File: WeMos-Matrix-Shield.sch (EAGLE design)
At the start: 16 parts, among them CN1 1X4-BIG, J2 POWER_JACKPTH, U1 LDR, U2 DS18B20, X1 SPTAF_25.0MM

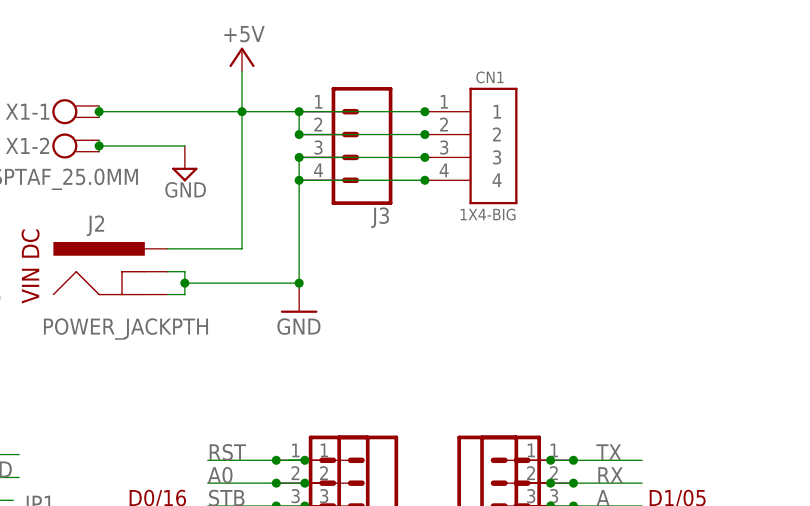
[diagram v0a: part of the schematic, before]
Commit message: Updated to V1.5
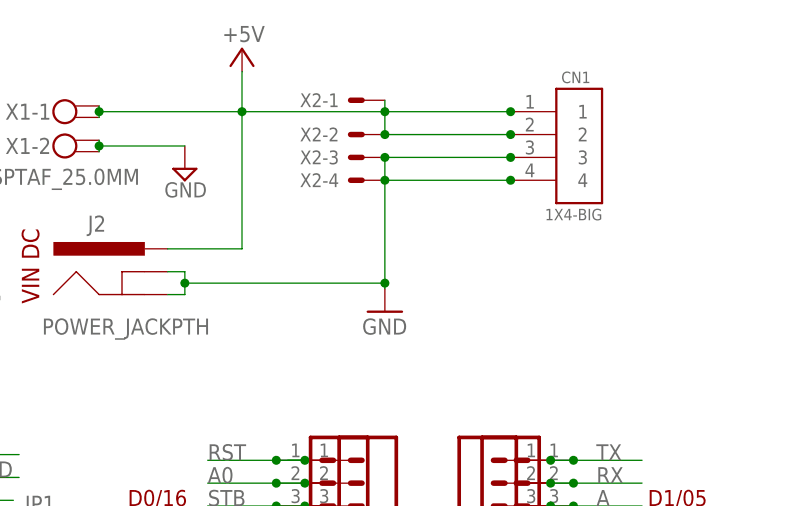
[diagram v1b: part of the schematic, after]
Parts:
- removed J3: (no value), SparkFun-Connectors:CONN_04SCREW
- added X2: (no value), con-molex:KK-156-4
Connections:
- net 5V: now also X2-1.S, X2-2.S; no longer J3.1, J3.2
- net GND: now also X2-3.S, X2-4.S; no longer J3.3, J3.4
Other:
- moved on the sheet: CN1

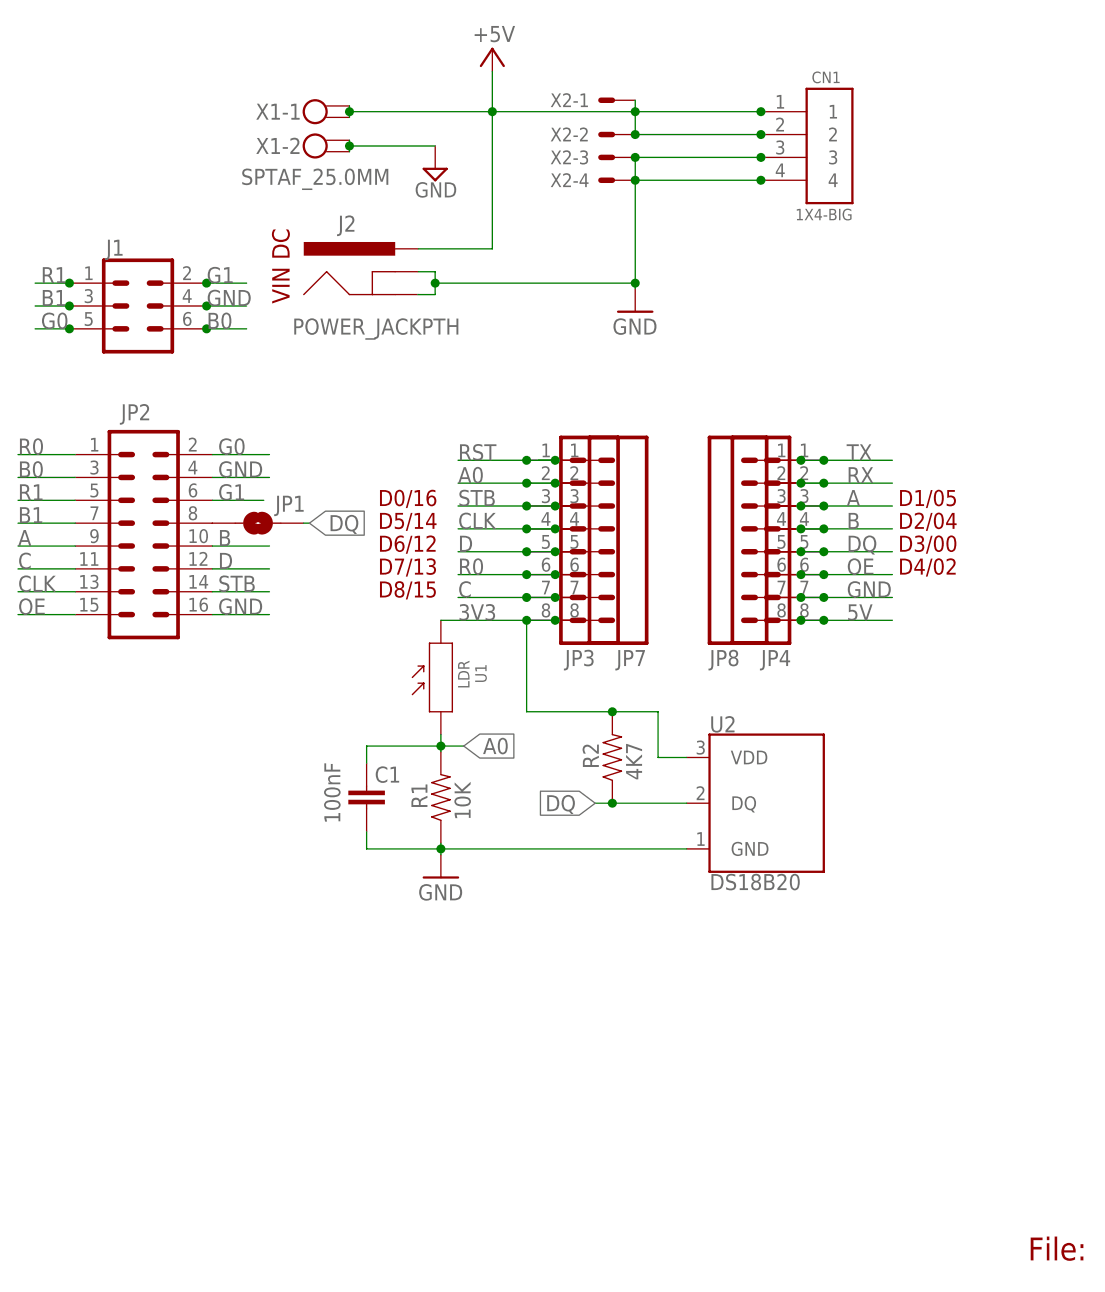
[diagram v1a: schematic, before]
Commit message: Updated to V1.6
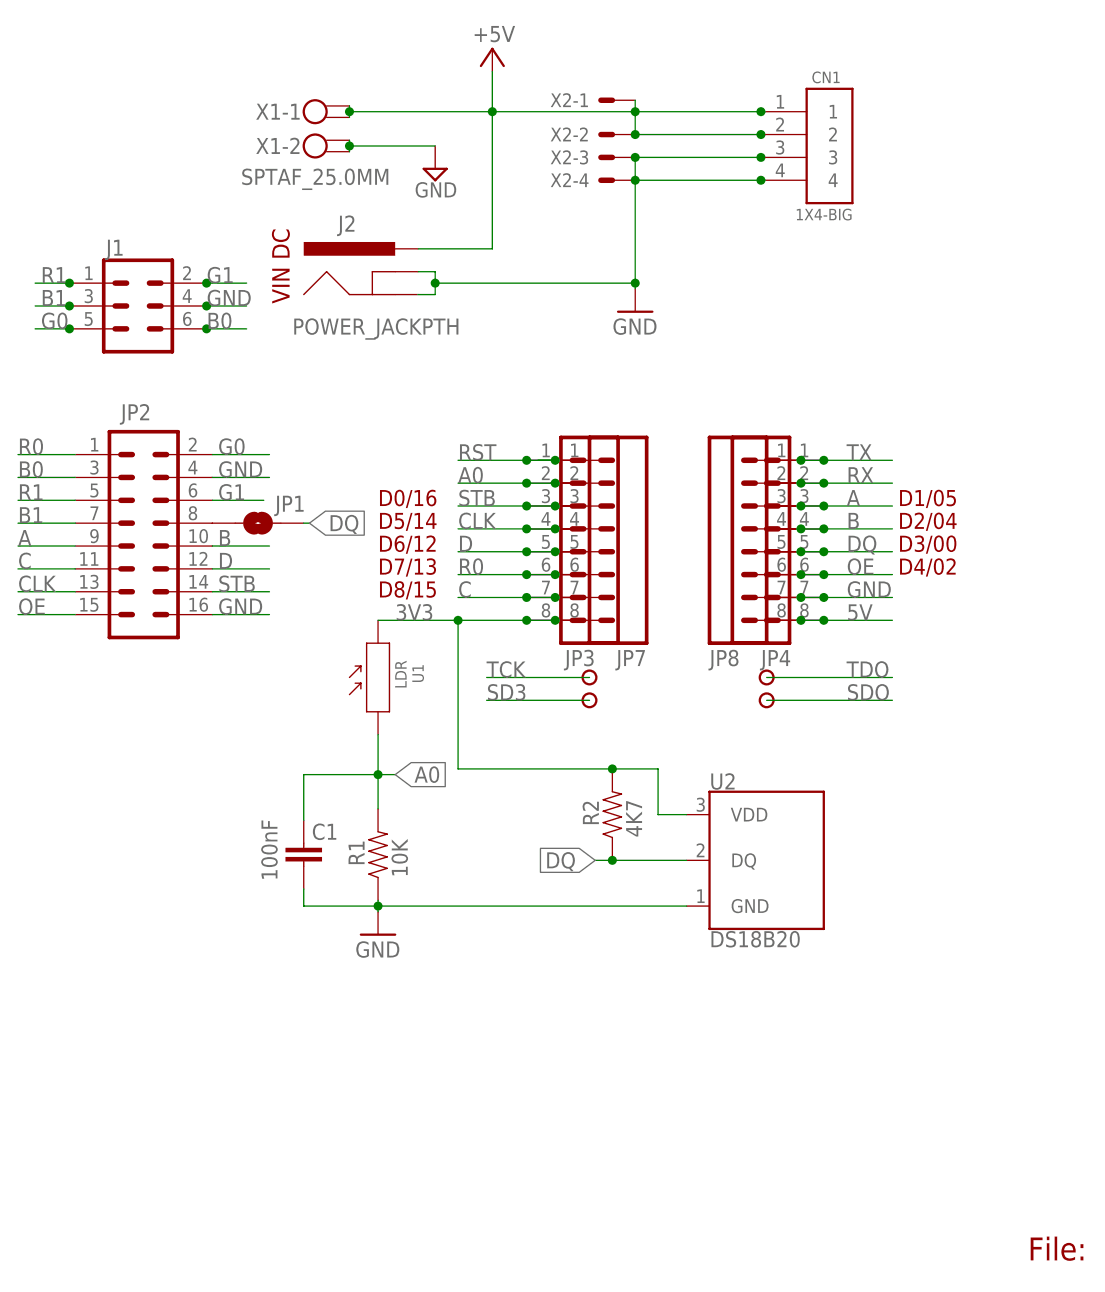
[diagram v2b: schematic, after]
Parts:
- added VIN1, VIN2, VIN3, VIN4: PADNORMAL, _c2h:PADNORMAL
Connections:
- new net SD3: VIN4.1
- new net SDO: VIN2.1
- new net TCK: VIN3.1
- new net TDO: VIN1.1
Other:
- moved on the sheet: C1, R1, R2, U1, U2
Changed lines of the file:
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@@
 <part name="NAME" library="SparkFun-Aesthetics" deviceset="FRAME-A4L" device="" value="Value">
 <attribute name="CNAME" value="ESP8266 Wemos Matrix Shield"/>
-<attribute name="CREVISION" value="1.5"/>
+<attribute name="CREVISION" value="1.6"/>
 <attribute name="DESIGNER" value="Charles-Henri Hallard"/>
 </part>
@@
 <part name="JP1" library="SparkFun-Jumpers" deviceset="JUMPER-SMT_2_NO" device="_NO-SILK" value="JUMPER-SMT_2_NO_NO-SILK"/>
 <part name="X2" library="con-molex" deviceset="KK-156-4" device=""/>
+<part name="VIN1" library="_c2h" deviceset="PAD" device="NORMAL"/>
+<part name="VIN2" library="_c2h" deviceset="PAD" device="NORMAL"/>
+<part name="VIN3" library="_c2h" deviceset="PAD" device="NORMAL"/>
+<part name="VIN4" library="_c2h" deviceset="PAD" device="NORMAL"/>
 </parts>
 <sheets>
@@
 </instance>
 <instance part="GND1" gate="1" x="145.415" y="121.92"/>
-<instance part="U1" gate="G$1" x="123.825" y="81.28" smashed="yes" rot="R90">
-<attribute name="VALUE" x="125.73" y="83.185" size="1.27" layer="96" ratio="10" rot="R270"/>
-<attribute name="NAME" x="128.905" y="80.645" size="1.27" layer="95" ratio="10" rot="R90"/>
-</instance>
-<instance part="R1" gate="G$1" x="123.825" y="67.945" smashed="yes" rot="R90">
-<attribute name="NAME" x="122.3264" y="66.675" size="1.778" layer="95" rot="R90"/>
-<attribute name="VALUE" x="127.127" y="65.405" size="1.778" layer="96" rot="R90"/>
-</instance>
-<instance part="GND2" gate="1" x="123.825" y="59.055"/>
-<instance part="C1" gate="G$1" x="115.57" y="66.675" smashed="yes">
-<attribute name="NAME" x="116.459" y="69.596" size="1.778" layer="95"/>
-<attribute name="VALUE" x="112.649" y="65.024" size="1.778" layer="96" rot="R90"/>
-</instance>
-<instance part="U2" gate="G$1" x="161.29" y="67.31"/>
-<instance part="R2" gate="G$1" x="142.875" y="72.39" smashed="yes" rot="R90">
-<attribute name="NAME" x="141.3764" y="71.12" size="1.778" layer="95" rot="R90"/>
-<attribute name="VALUE" x="146.177" y="69.85" size="1.778" layer="96" rot="R90"/>
+<instance part="U1" gate="G$1" x="116.84" y="81.28" smashed="yes" rot="R90">
+<attribute name="VALUE" x="118.745" y="83.185" size="1.27" layer="96" ratio="10" rot="R270"/>
+<attribute name="NAME" x="121.92" y="80.645" size="1.27" layer="95" ratio="10" rot="R90"/>
+</instance>
+<instance part="R1" gate="G$1" x="116.84" y="61.595" smashed="yes" rot="R90">
+<attribute name="NAME" x="115.3414" y="60.325" size="1.778" layer="95" rot="R90"/>
+<attribute name="VALUE" x="120.142" y="59.055" size="1.778" layer="96" rot="R90"/>
+</instance>
+<instance part="GND2" gate="1" x="116.84" y="52.705"/>
+<instance part="C1" gate="G$1" x="108.585" y="60.325" smashed="yes">
+<attribute name="NAME" x="109.474" y="63.246" size="1.778" layer="95"/>
+<attribute name="VALUE" x="105.664" y="58.674" size="1.778" layer="96" rot="R90"/>
+</instance>
+<instance part="U2" gate="G$1" x="161.29" y="60.96"/>
+<instance part="R2" gate="G$1" x="142.875" y="66.04" smashed="yes" rot="R90">
+<attribute name="NAME" x="141.3764" y="64.77" size="1.778" layer="95" rot="R90"/>
+<attribute name="VALUE" x="146.177" y="63.5" size="1.778" layer="96" rot="R90"/>
 </instance>
 <instance part="JP1" gate="G$1" x="103.505" y="98.425" smashed="yes">
@@
 <instance part="X2" gate="-3" x="142.875" y="139.065" rot="R180"/>
 <instance part="X2" gate="-4" x="142.875" y="136.525" rot="R180"/>
+<instance part="VIN1" gate="G$1" x="160.02" y="81.28"/>
+<instance part="VIN2" gate="G$1" x="160.02" y="78.74"/>
+<instance part="VIN3" gate="G$1" x="140.335" y="81.28"/>
+<instance part="VIN4" gate="G$1" x="140.335" y="78.74"/>
 </instances>
 <busses>
@@
 <pinref part="R1" gate="G$1" pin="1"/>
 <pinref part="GND2" gate="1" pin="GND"/>
-<wire x1="123.825" y1="61.595" x2="123.825" y2="62.23" width="0.1524" layer="91"/>
+<wire x1="116.84" y1="55.245" x2="116.84" y2="55.88" width="0.1524" layer="91"/>
 <pinref part="C1" gate="G$1" pin="2"/>
-<wire x1="123.825" y1="62.23" x2="123.825" y2="62.865" width="0.1524" layer="91"/>
-<wire x1="123.825" y1="62.23" x2="115.57" y2="62.23" width="0.1524" layer="91"/>
-<wire x1="115.57" y1="62.23" x2="115.57" y2="64.135" width="0.1524" layer="91"/>
-<junction x="123.825" y="62.23"/>
+<wire x1="116.84" y1="55.88" x2="116.84" y2="56.515" width="0.1524" layer="91"/>
+<wire x1="116.84" y1="55.88" x2="108.585" y2="55.88" width="0.1524" layer="91"/>
+<wire x1="108.585" y1="55.88" x2="108.585" y2="57.785" width="0.1524" layer="91"/>
+<junction x="116.84" y="55.88"/>
 <pinref part="U2" gate="G$1" pin="GND"/>
-<wire x1="151.13" y1="62.23" x2="123.825" y2="62.23" width="0.1524" layer="91"/>
+<wire x1="151.13" y1="55.88" x2="116.84" y2="55.88" width="0.1524" layer="91"/>
 </segment>
 </net>
@@
 <segment>
 <pinref part="JP3" gate="G$1" pin="8"/>
-<label x="125.73" y="87.63" size="1.778" layer="95"/>
+<label x="118.745" y="87.63" size="1.778" layer="95"/>
 <pinref part="JP7" gate="G$1" pin="8"/>
 <junction x="136.525" y="87.63"/>
-<wire x1="133.35" y1="87.63" x2="123.825" y2="87.63" width="0.1524" layer="91"/>
+<wire x1="133.35" y1="87.63" x2="125.73" y2="87.63" width="0.1524" layer="91"/>
+<wire x1="125.73" y1="87.63" x2="116.84" y2="87.63" width="0.1524" layer="91"/>
 <wire x1="136.525" y1="87.63" x2="133.35" y2="87.63" width="0.1524" layer="91"/>
 <pinref part="U1" gate="G$1" pin="P$2"/>
 <junction x="133.35" y="87.63"/>
 <pinref part="U2" gate="G$1" pin="VDD"/>
-<wire x1="151.13" y1="72.39" x2="147.955" y2="72.39" width="0.1524" layer="91"/>
-<wire x1="147.955" y1="72.39" x2="147.955" y2="77.47" width="0.1524" layer="91"/>
+<wire x1="151.13" y1="66.04" x2="147.955" y2="66.04" width="0.1524" layer="91"/>
+<wire x1="147.955" y1="66.04" x2="147.955" y2="71.12" width="0.1524" layer="91"/>
 <pinref part="R2" gate="G$1" pin="2"/>
-<wire x1="147.955" y1="77.47" x2="142.875" y2="77.47" width="0.1524" layer="91"/>
-<wire x1="142.875" y1="77.47" x2="133.35" y2="77.47" width="0.1524" layer="91"/>
-<wire x1="133.35" y1="77.47" x2="133.35" y2="87.63" width="0.1524" layer="91"/>
-<junction x="142.875" y="77.47"/>
+<wire x1="147.955" y1="71.12" x2="142.875" y2="71.12" width="0.1524" layer="91"/>
+<wire x1="142.875" y1="71.12" x2="125.73" y2="71.12" width="0.1524" layer="91"/>
+<junction x="142.875" y="71.12"/>
+<wire x1="125.73" y1="71.12" x2="125.73" y2="87.63" width="0.1524" layer="91"/>
+<junction x="125.73" y="87.63"/>
 </segment>
 </net>
@@
 <segment>
 <pinref part="U1" gate="G$1" pin="P$1"/>
-<wire x1="123.825" y1="74.93" x2="123.825" y2="73.66" width="0.1524" layer="91"/>
+<wire x1="116.84" y1="74.93" x2="116.84" y2="70.485" width="0.1524" layer="91"/>
 <pinref part="R1" gate="G$1" pin="2"/>
-<wire x1="123.825" y1="73.66" x2="123.825" y2="73.025" width="0.1524" layer="91"/>
-<wire x1="123.825" y1="73.66" x2="126.365" y2="73.66" width="0.1524" layer="91"/>
-<label x="126.365" y="73.66" size="1.778" layer="95" xref="yes"/>
-<junction x="123.825" y="73.66"/>
+<wire x1="116.84" y1="70.485" x2="116.84" y2="66.675" width="0.1524" layer="91"/>
+<wire x1="116.84" y1="70.485" x2="118.745" y2="70.485" width="0.1524" layer="91"/>
+<label x="118.745" y="70.485" size="1.778" layer="95" xref="yes"/>
+<junction x="116.84" y="70.485"/>
 <pinref part="C1" gate="G$1" pin="1"/>
-<wire x1="123.825" y1="73.66" x2="115.57" y2="73.66" width="0.1524" layer="91"/>
-<wire x1="115.57" y1="73.66" x2="115.57" y2="71.755" width="0.1524" layer="91"/>
+<wire x1="116.84" y1="70.485" x2="108.585" y2="70.485" width="0.1524" layer="91"/>
+<wire x1="108.585" y1="70.485" x2="108.585" y2="65.405" width="0.1524" layer="91"/>
 </segment>
 </net>
@@
 <segment>
 <pinref part="U2" gate="G$1" pin="DQ"/>
-<wire x1="151.13" y1="67.31" x2="142.875" y2="67.31" width="0.1524" layer="91"/>
+<wire x1="151.13" y1="60.96" x2="142.875" y2="60.96" width="0.1524" layer="91"/>
 <pinref part="R2" gate="G$1" pin="1"/>
-<junction x="142.875" y="67.31"/>
-<wire x1="142.875" y1="67.31" x2="140.97" y2="67.31" width="0.1524" layer="91"/>
-<label x="140.97" y="67.31" size="1.778" layer="95" rot="R180" xref="yes"/>
+<junction x="142.875" y="60.96"/>
+<wire x1="142.875" y1="60.96" x2="140.97" y2="60.96" width="0.1524" layer="91"/>
+<label x="140.97" y="60.96" size="1.778" layer="95" rot="R180" xref="yes"/>
 </segment>
 <segment>
@@
 </segment>
 </net>
+<net name="TDO" class="0">
+<segment>
+<pinref part="VIN1" gate="G$1" pin="1"/>
+<wire x1="160.02" y1="81.28" x2="173.99" y2="81.28" width="0.1524" layer="91"/>
+<label x="168.91" y="81.28" size="1.778" layer="95"/>
+</segment>
+</net>
+<net name="SDO" class="0">
+<segment>
+<pinref part="VIN2" gate="G$1" pin="1"/>
+<wire x1="160.02" y1="78.74" x2="173.99" y2="78.74" width="0.1524" layer="91"/>
+<label x="168.91" y="78.74" size="1.778" layer="95"/>
+</segment>
+</net>
+<net name="TCK" class="0">
+<segment>
+<wire x1="140.335" y1="81.28" x2="128.905" y2="81.28" width="0.1524" layer="91"/>
+<label x="128.905" y="81.28" size="1.778" layer="95"/>
+<pinref part="VIN3" gate="G$1" pin="1"/>
+</segment>
+</net>
+<net name="SD3" class="0">
+<segment>
+<wire x1="140.335" y1="78.74" x2="128.905" y2="78.74" width="0.1524" layer="91"/>
+<label x="128.905" y="78.74" size="1.778" layer="95"/>
+<pinref part="VIN4" gate="G$1" pin="1"/>
+</segment>
+</net>
